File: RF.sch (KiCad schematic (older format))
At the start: 43 parts, among them Q1 2N7002, Q2 IRLML2060, U4 LM4562, U5 74AHCT1G00, U6 SN74CBT3253, U7 Filter

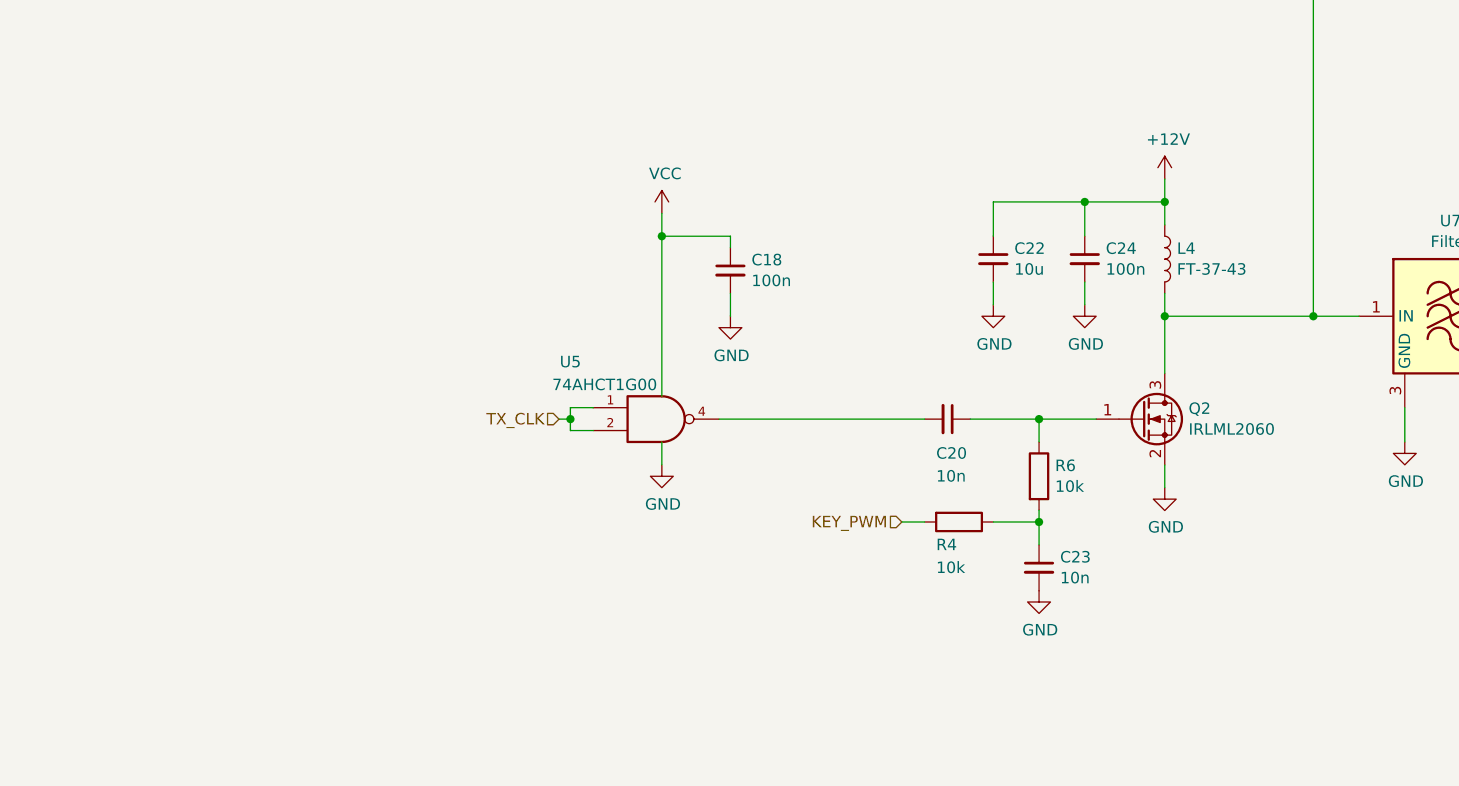
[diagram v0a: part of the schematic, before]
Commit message: Work on PCB
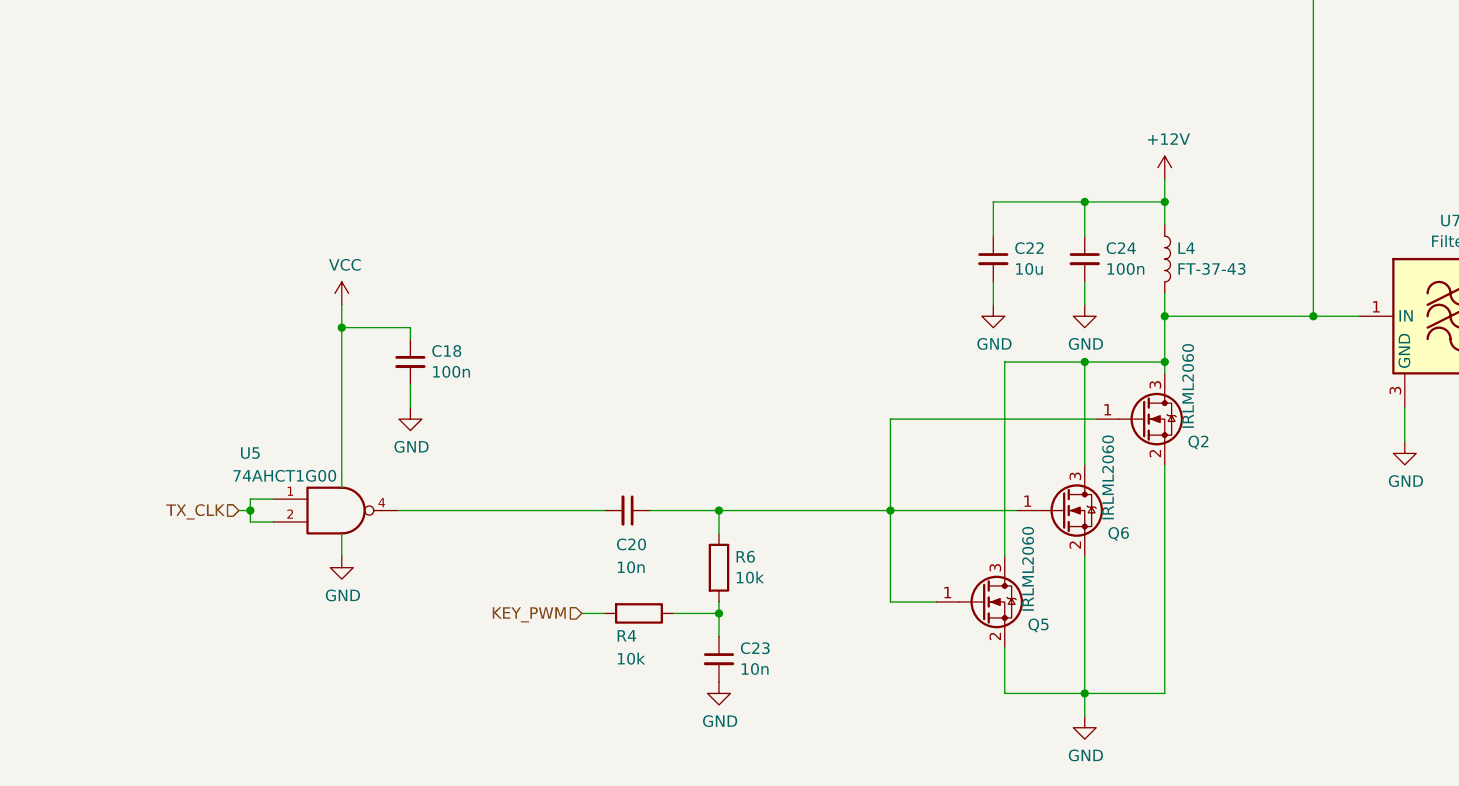
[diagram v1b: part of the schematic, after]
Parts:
- added Q5, Q6: IRLML2060, Package_TO_SOT_SMD:SOT-23, symbol Transistor_FET:IRLML2060
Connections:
- net GND: now also Q5.2 (S), Q6.2 (S)
- net at C16.2, L4.2, Q2.3 (D)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: now also Q5.3 (D), Q6.3 (D)
- net at C20.1, Q2.1 (G), R6.1: now also Q5.1 (G), Q6.1 (G)
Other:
- moved on the sheet: C18, C20, C23, R4, R6, U5
